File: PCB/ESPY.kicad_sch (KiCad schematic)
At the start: 91 parts, among them J1 Conn_01x15_Socket, J2 USB_C_Receptacle_USB2.0_16P, J3 USB_C_Receptacle_USB2.0_16P, J5 Conn_01x15_Socket, J6 Conn_01x20_Pin, J7 Conn_01x08_Pin, J9 Conn_01x16_Pin, SW1 SW_DPST_x2, U2 TLV62569ADRL, U4 TLV62569ADRL, U5 CH334R, Y1 40Mhz(+/-10ppm), Y3 12Mhz

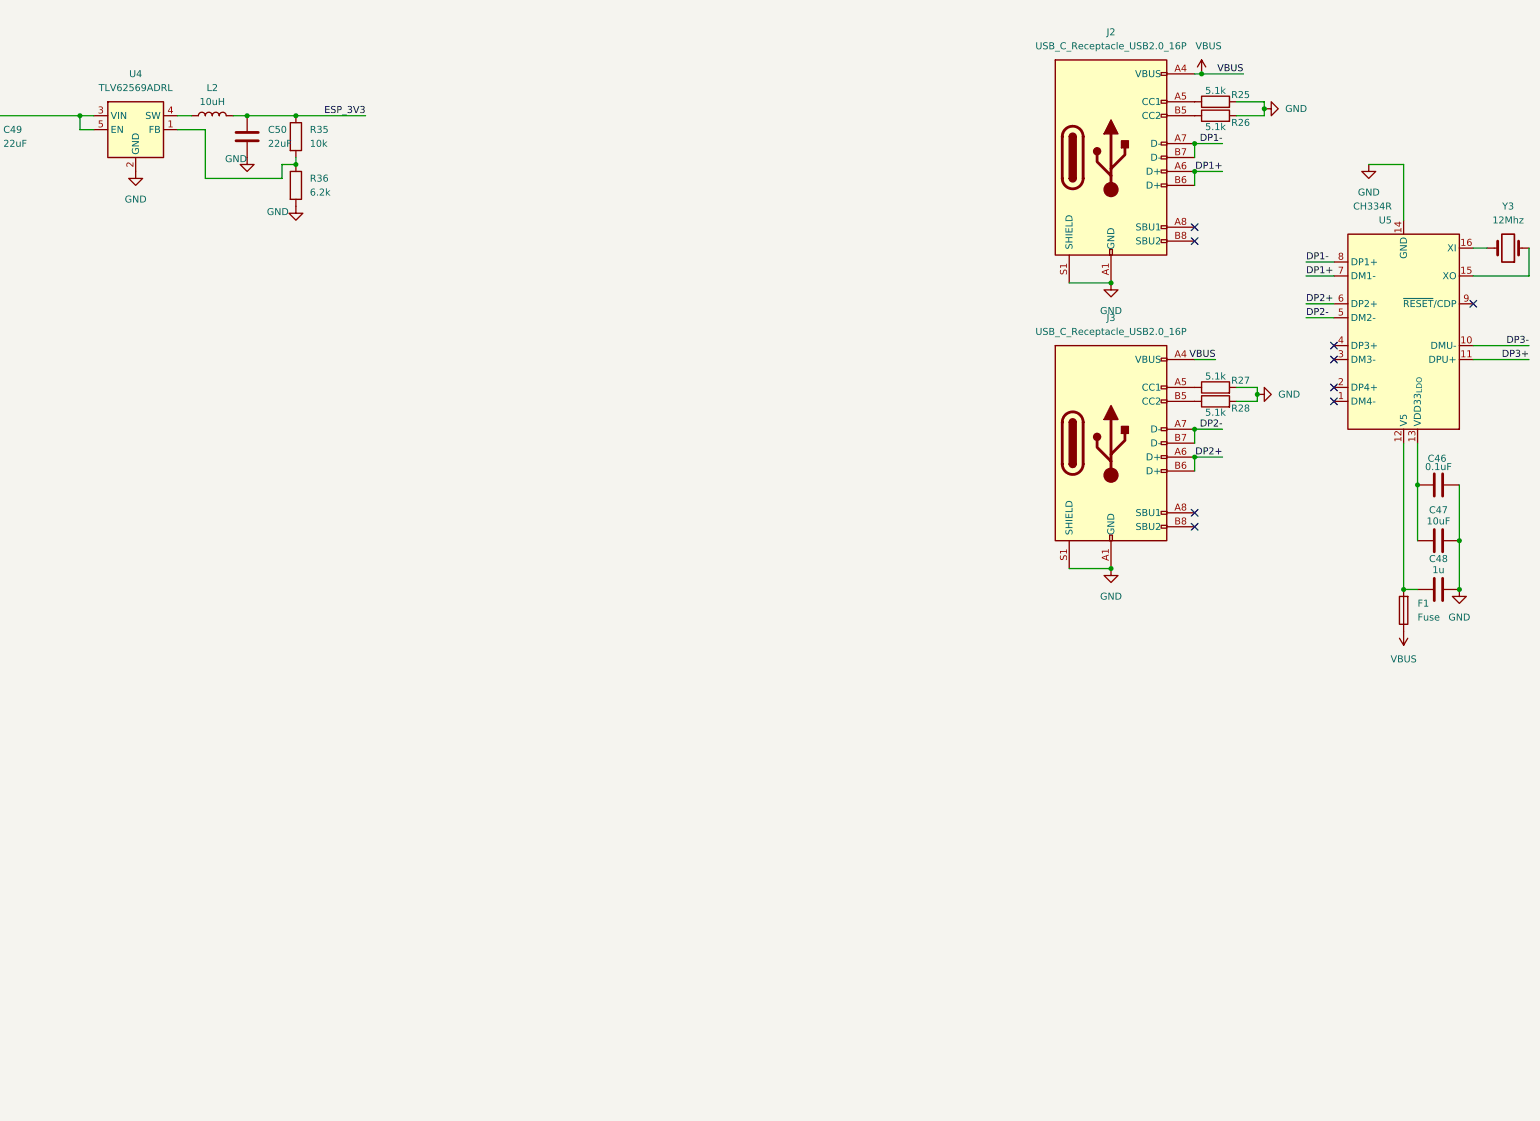
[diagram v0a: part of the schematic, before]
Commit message: files saved
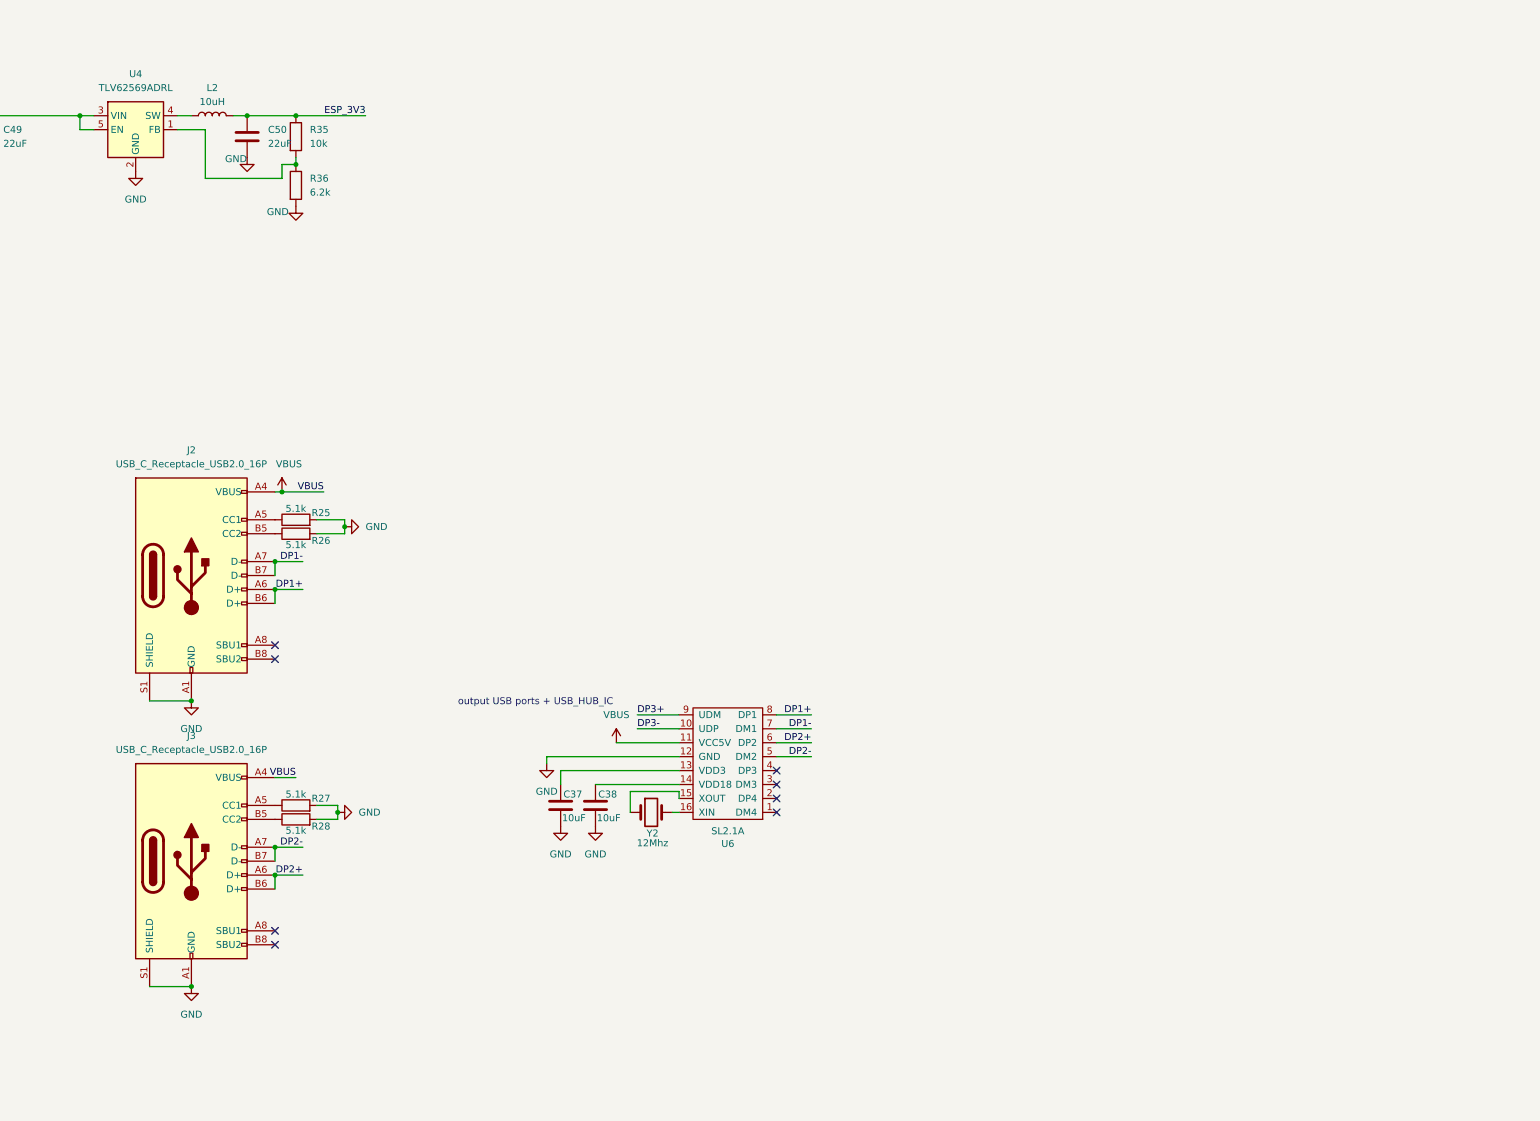
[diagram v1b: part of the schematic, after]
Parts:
- removed C46: 0.1uF, Capacitor_SMD:C_0402_1005Metric, symbol Device:C
- removed C47: 10uF, Capacitor_SMD:C_0402_1005Metric, symbol Device:C
- removed C48: 1u, Capacitor_SMD:C_0402_1005Metric, symbol Device:C
- removed F1: Fuse, Fuse:Fuse_0402_1005Metric, symbol Device:Fuse
- removed U5: CH334R, Package_SO:QSOP-16_3.9x4.9mm_P0.635mm, symbol Interface_USB:CH334R
- removed Y3: 12Mhz, Crystal:Crystal_SMD_0603-2Pin_6.0x3.5mm, symbol Device:Crystal
- added C37, C38: 10uF, Capacitor_SMD:C_0402_1005Metric, symbol Device:C
- added U6: SL2.1A, Package_SO:SOIC-16_4.55x10.3mm_P1.27mm, symbol SL2.1A:SL2.1A
- added Y2: 12Mhz, Crystal:Crystal_SMD_3215-2Pin_3.2x1.5mm, symbol Device:Crystal
- J1, J5: footprint Connector_FFC-FPC:Amphenol_F32Q-1A7x1-11015_1x15-1MP_P0.5mm_Horizontal -> Connector_FFC-FPC:Molex_502244-1530_1x15-1MP_P0.5mm_Horizontal
- L2: footprint Inductor_SMD:L_0402_1005Metric -> Inductor_SMD:L_0603_1608Metric
- W25Q512JVFIQ1: footprint Package_SON:WSON-8-1EP_6x5mm_P1.27mm_EP3.4x4.3mm -> Package_SO:SOIC-16W_7.5x10.3mm_P1.27mm
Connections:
- net DP1+: now also U6.8 (DP1)
- net DP1-: now also U6.7 (DM1)
- net DP2+: now also U6.6 (DP2)
- net DP2-: now also U6.5 (DM2)
- net DP3+: now also U6.9 (UDM)
- net DP3-: now also U6.10 (UDP)
- net GND: now also C37.2, C38.2, U6.12 (GND)
- net VBUS: now also U6.11 (VCC5V)
- new net: C38.1, U6.14 (VDD18)
- new net: U6.15 (XOUT), Y2.1
- new net: U6.16 (XIN), Y2.2
- new net: C37.1, U6.13 (VDD3)
- no-connect marks 12 -> 11
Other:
- note added: "output USB ports + USB_HUB_IC"
- moved on the sheet: J2, J3, R25, R26, R27, R28
